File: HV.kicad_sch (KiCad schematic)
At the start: 70 parts, among them J1 HVConnector, U1 TLV9002QDRQ1

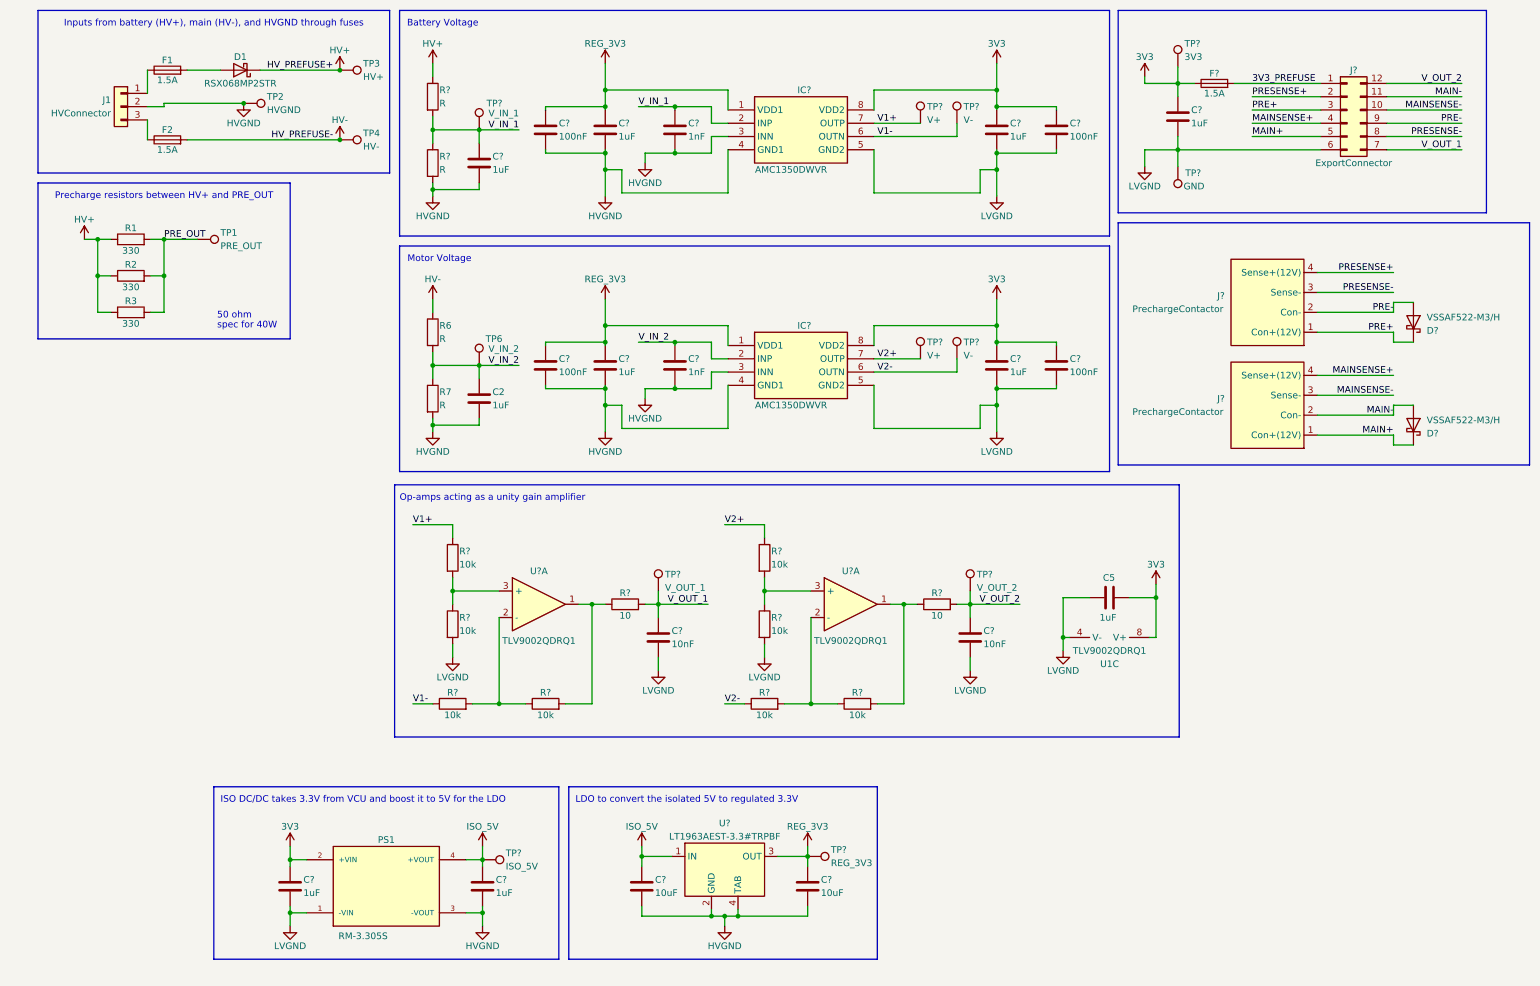
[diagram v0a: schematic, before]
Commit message: CAN nano & CAN debug nano
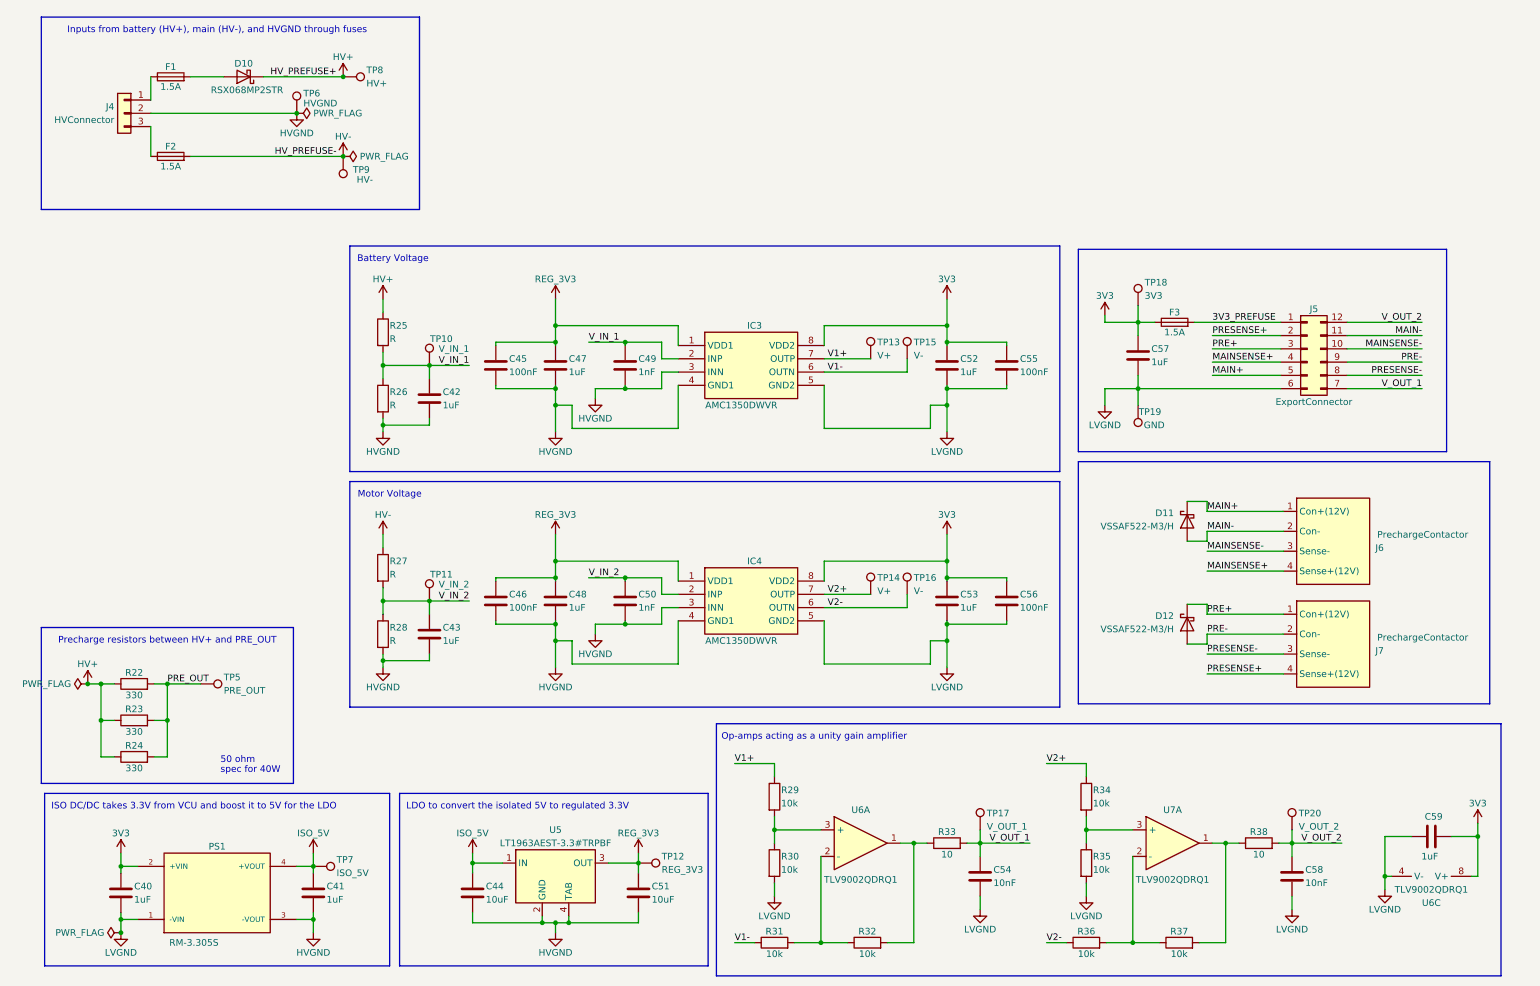
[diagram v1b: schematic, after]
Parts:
- gave numbers to parts that had none: 52
- renumbered C2 to C43, C5 to C59, D1 to D10, J1 to J4, R1 to R22, R2 to R23, R3 to R24, R6 to R27, R7 to R28, TP6 to TP11, TP1 to TP5, TP2 to TP6, TP3 to TP8, TP4 to TP9, U1 to U6
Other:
- moved on the sheet: C40, C41, C42, C43, C44, C45, C46, C47, C48, C49, C50, C51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
